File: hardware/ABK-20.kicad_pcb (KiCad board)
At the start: 2 copper layers, 75 x 80 mm, 72 parts, among them J1 CONN_01X04, J2 CONN_01X04, J4 Con_3-5V, J5 USB_C_6P, J6 Sync_Jumper, SW1 SW_SPST, SW2 SW_Push_LED, SW3 SW_SPDT_MSM, SW4 SW_Push, U1 ATTINY85-20SU, U2 PAM8002, U3 7805

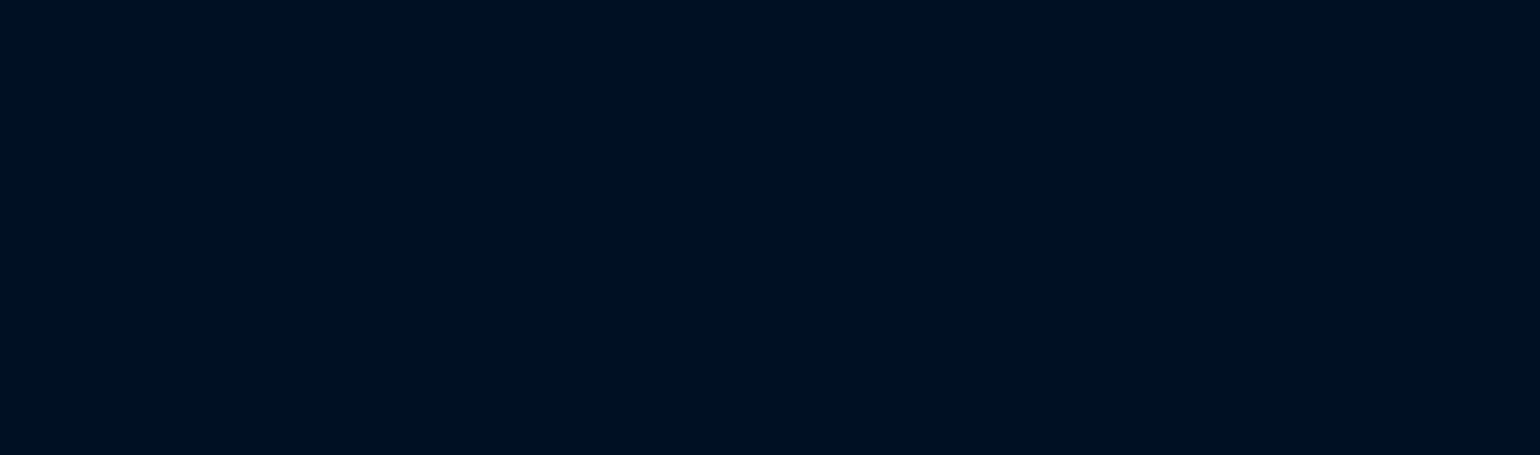
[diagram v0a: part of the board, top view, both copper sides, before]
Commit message: deleted files
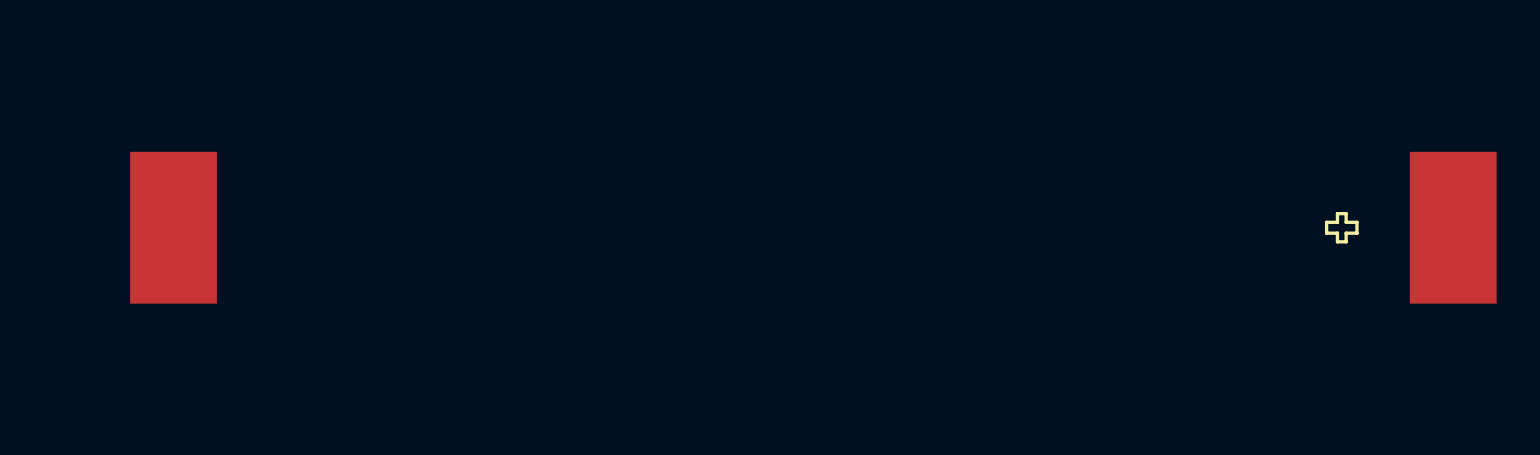
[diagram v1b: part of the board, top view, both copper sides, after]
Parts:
- added BT2: Battery_Cell, 8Bitmixtape_reworked:BAT_Holder_AAA-new_noHole, F.Cu at (200.5, 66.4)
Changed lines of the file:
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@@
+		)
+	)
+	(footprint "8Bitmixtape_reworked:BAT_Holder_AAA-new_noHole"
+		(layer "F.Cu")
+		(at 200.533 66.421)
+		(property "Reference" "BT2"
+			(at 0 -3.81 0)
+			(layer "Eco2.User")
+			(effects
+				(font
+					(size 1 1)
+					(thickness 0.15)
+				)
+			)
+		)
+		(property "Value" "Battery_Cell"
+			(at 0.254 3.81 0)
+			(layer "Eco2.User")
+			(effects
+				(font
+					(size 1 1)
+					(thickness 0.15)
+				)
+			)
+		)
+		(property "Datasheet" ""
+			(at 0 0 0)
+			(layer "F.Fab")
+			(hide yes)
+			(effects
+				(font
+					(size 1.27 1.27)
+					(thickness 0.15)
+				)
+			)
+		)
+		(property "Description" ""
+			(at 0 0 0)
+			(layer "F.Fab")
+			(hide yes)
+			(effects
+				(font
+					(size 1.27 1.27)
+					(thickness 0.15)
+				)
+			)
+		)
+		(attr through_hole)
+		(fp_line
+			(start 23.662 0.134)
+			(end 23.662 -0.366)
+			(stroke
+				(width 0.1524)
+				(type solid)
+			)
+			(layer "F.SilkS")
+		)
+		(fp_line
+			(start 23.662 0.134)
+			(end 24.162 0.134)
+			(stroke
+				(width 0.1524)
+				(type solid)
+			)
+			(layer "F.SilkS")
+		)
+		(fp_line
+			(start 24.162 -0.766)
+			(end 24.562 -0.766)
+			(stroke
+				(width 0.1524)
+				(type solid)
+			)
+			(layer "F.SilkS")
+		)
+		(fp_line
+			(start 24.162 -0.366)
+			(end 23.662 -0.366)
+			(stroke
+				(width 0.1524)
+				(type solid)
+			)
+			(layer "F.SilkS")
+		)
+		(fp_line
+			(start 24.162 -0.366)
+			(end 24.162 -0.766)
+			(stroke
+				(width 0.1524)
+				(type solid)
+			)
+			(layer "F.SilkS")
+		)
+		(fp_line
+			(start 24.162 0.534)
+			(end 24.162 0.134)
+			(stroke
+				(width 0.1524)
+				(type solid)
+			)
+			(layer "F.SilkS")
+		)
+		(fp_line
+			(start 24.562 -0.766)
+			(end 24.562 -0.366)
+			(stroke
+				(width 0.1524)
+				(type solid)
+			)
+			(layer "F.SilkS")
+		)
+		(fp_line
+			(start 24.562 -0.366)
+			(end 25.062 -0.366)
+			(stroke
+				(width 0.1524)
+				(type solid)
+			)
+			(layer "F.SilkS")
+		)
+		(fp_line
+			(start 24.562 0.134)
+			(end 24.562 0.534)
+			(stroke
+				(width 0.1524)
+				(type solid)
+			)
+			(layer "F.SilkS")
+		)
+		(fp_line
+			(start 24.562 0.534)
+			(end 24.162 0.534)
+			(stroke
+				(width 0.1524)
+				(type solid)
+			)
+			(layer "F.SilkS")
+		)
+		(fp_line
+			(start 25.062 -0.366)
+			(end 25.062 0.134)
+			(stroke
+				(width 0.1524)
+				(type solid)
+			)
+			(layer "F.SilkS")
+		)
+		(fp_line
+			(start 25.062 0.134)
+			(end 24.562 0.134)
+			(stroke
+				(width 0.1524)
+				(type solid)
+			)
+			(layer "F.SilkS")
+		)
+		(fp_line
+			(start -27.18 -5.786)
+			(end -27.178 5.334)
+			(stroke
+				(width 0.15)
+				(type solid)
+			)
+			(layer "Eco2.User")
+		)
+		(fp_line
+			(start -27.18 -5.786)
+			(end 27.18 -5.786)
+			(stroke
+				(width 0.15)
+				(type solid)
+			)
+			(layer "Eco2.User")
+		)
+		(fp_line
+			(start -27.18 5.334)
+			(end 27.18 5.334)
+			(stroke
+				(width 0.15)
+				(type solid)
+			)
+			(layer "Eco2.User")
+		)
+		(fp_line
+			(start 27.178 5.334)
+			(end 27.18 -5.786)
+			(stroke
+				(width 0.15)
+				(type solid)
+			)
+			(layer "Eco2.User")
+		)
+		(fp_line
+			(start 31 -0.116)
+			(end -31 -0.116)
+			(stroke
+				(width 0.1524)
+				(type solid)
+			)
+			(layer "Eco2.User")
+		)
+		(pad "1" smd rect
+			(at 29.5 -0.116)
+			(size 4 7)
+			(layers "F.Cu" "F.Mask" "F.Paste")
+			(solder_mask_margin 0.01)
+		)
+		(pad "2" smd rect
+			(at -29.5 -0.116)
+			(size 4 7)
+			(layers "F.Cu" "F.Mask" "F.Paste")
+			(solder_mask_margin 0.01)
+		)
+		(embedded_fonts no)
+		(model "${KIPRJMOD}/3d_models/BatteryHolder_Keystone_2466_1xAAA.wrl"
+			(offset
+				(xyz 0 0 0)
+			)
+			(scale
+				(xyz 1 1 1)
+			)
+			(rotate
+				(xyz 0 0 0)
+			)
 		)
 	)
